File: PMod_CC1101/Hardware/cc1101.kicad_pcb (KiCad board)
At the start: 4 copper layers, 40.5 x 17 mm, 19 parts, among them J1 Conn_Coaxial, J2 Conn_02x06_Odd_Even, U1 CC1101RGPR

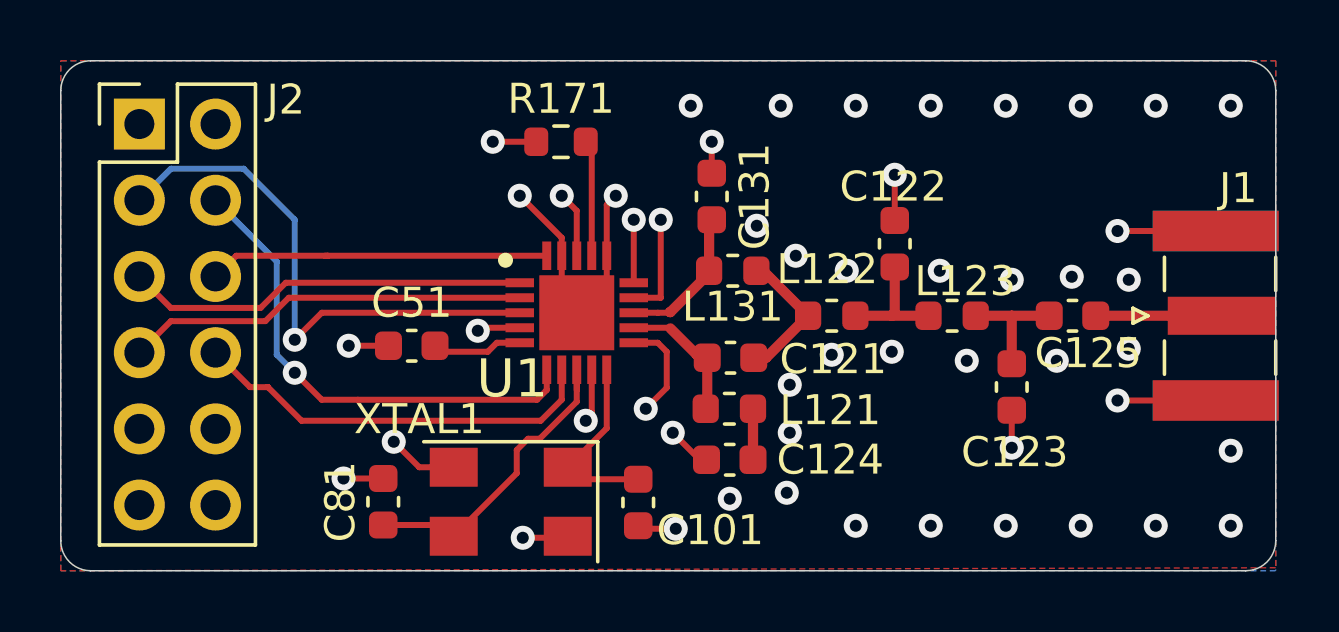
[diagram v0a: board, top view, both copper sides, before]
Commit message: add kicad7 pcb
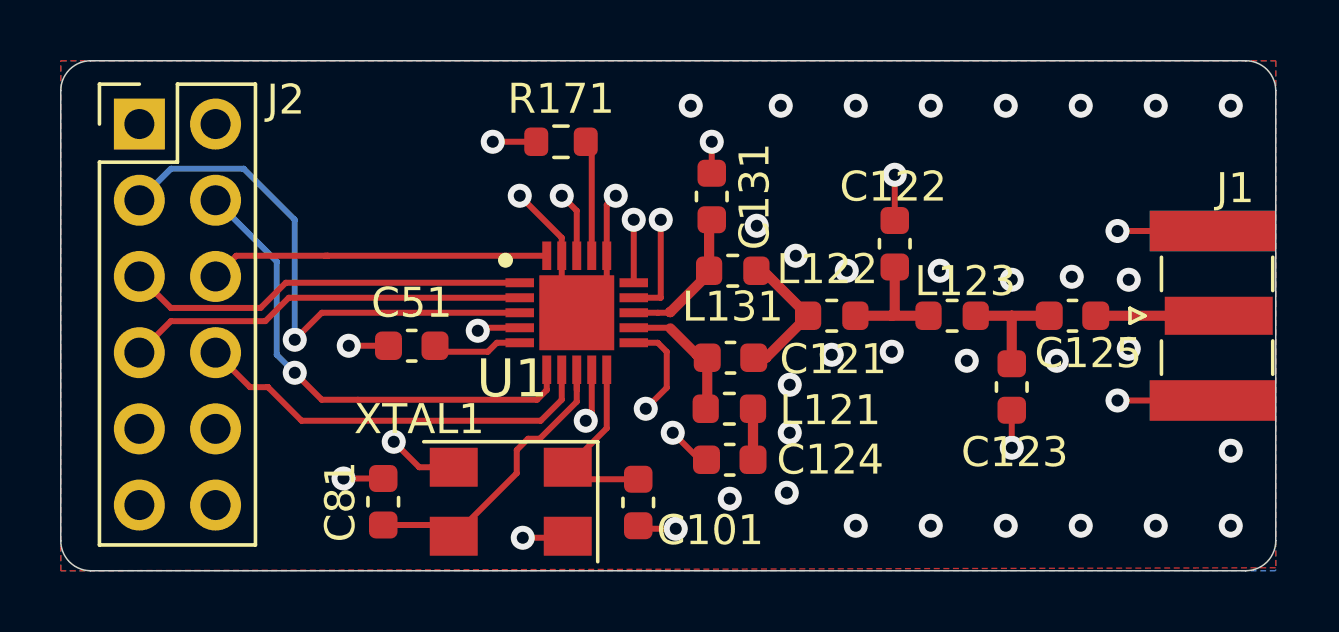
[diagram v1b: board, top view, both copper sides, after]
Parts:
- moved J1 0.10 mm to (169.4, 63.0)
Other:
- net class Default removed

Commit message: change logo designator
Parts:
- renumbered G*** to Logo1
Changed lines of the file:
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@@
     (at 153.35 63.5 180)
     (attr through_hole)
-    (fp_text reference "G***" (at 0 0) (layer "B.SilkS") hide
+    (fp_text reference "Logo1" (at 0 0) (layer "B.SilkS") hide
         (effects (font (size 1.524 1.524) (thickness 0.3)) (justify mirror))
     )

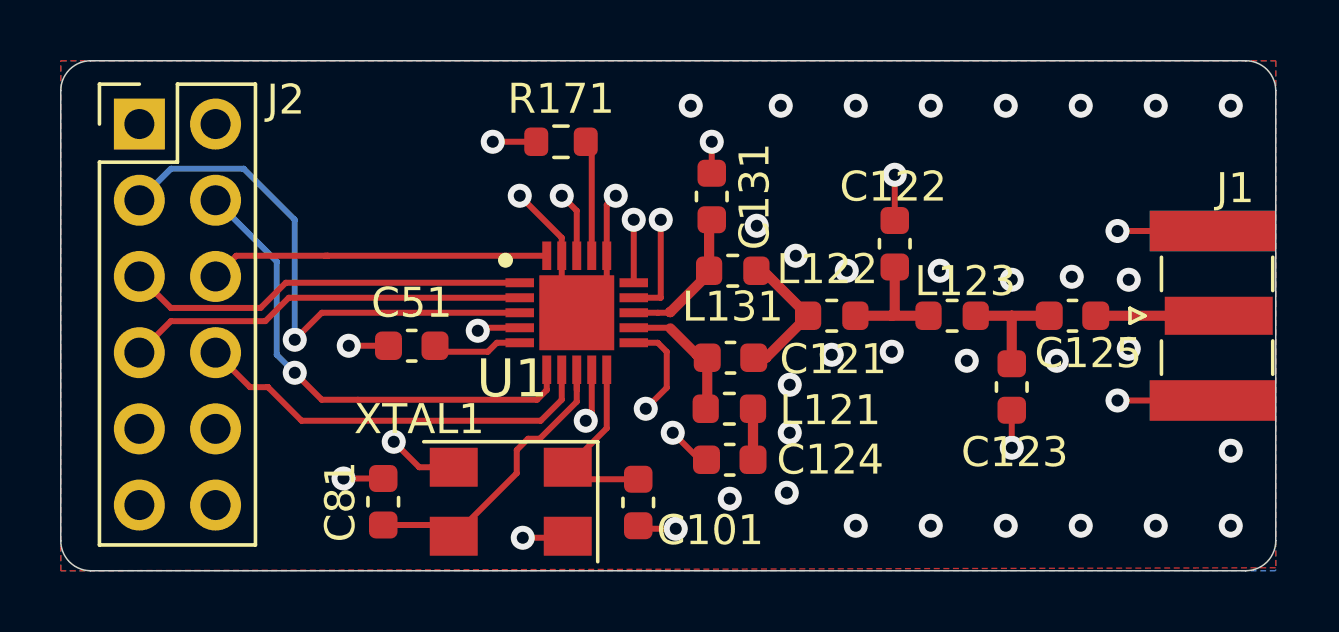
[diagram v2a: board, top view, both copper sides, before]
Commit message: update cc1101 center pad to pin 21
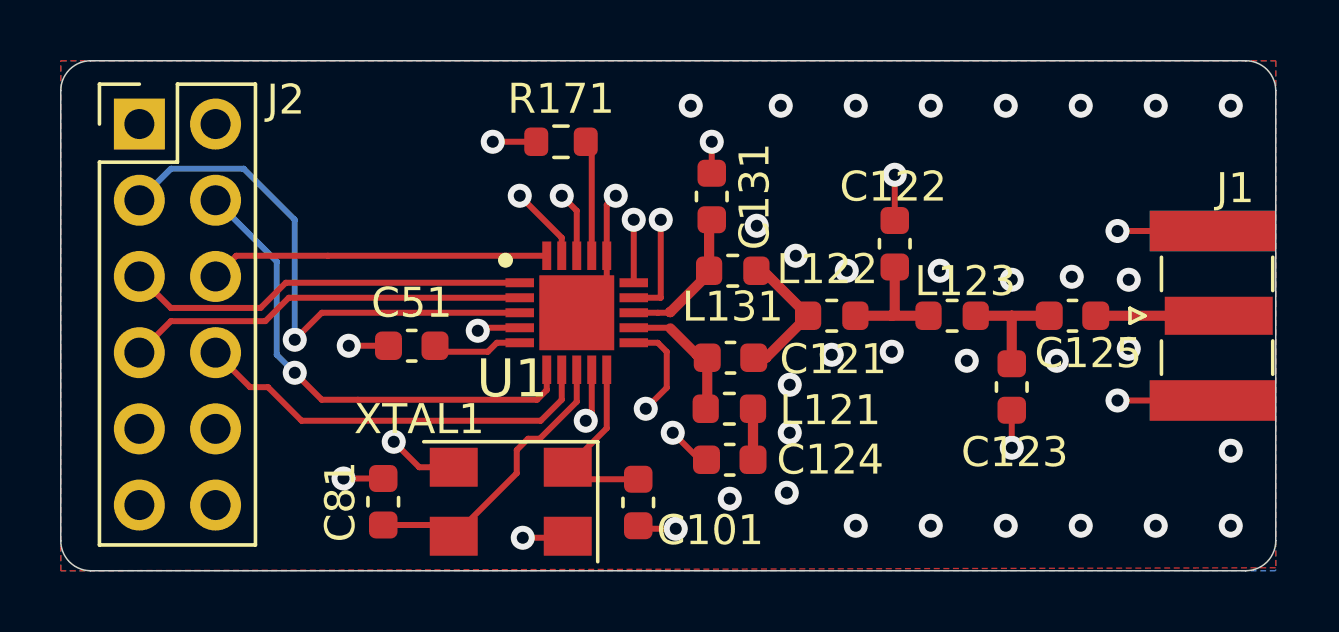
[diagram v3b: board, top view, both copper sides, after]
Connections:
- J2 pad 1: Net-(J2-Pad1) -> unconnected-(J2-Pin_1-Pad1)
- J2 pad 2: Net-(J2-Pad2) -> unconnected-(J2-Pin_2-Pad2)
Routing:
- net GND: track 31.0 -> 28.9 mm
- net Net-(U1-XOSC_Q1): track 10.7 -> 9.98 mm
